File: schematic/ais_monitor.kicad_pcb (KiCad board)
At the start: 2 copper layers, 109.5 x 72.5 mm, 73 parts, among them J1 Power Input (12/24), J2 GPS, Q1 Q_NMOS_DGS, SW1 Mute, U1 TPS73701, U2 LM321, U3 ADP2302ARDZ, U4 Pico, U5 PAM8302AAD, U6 feather

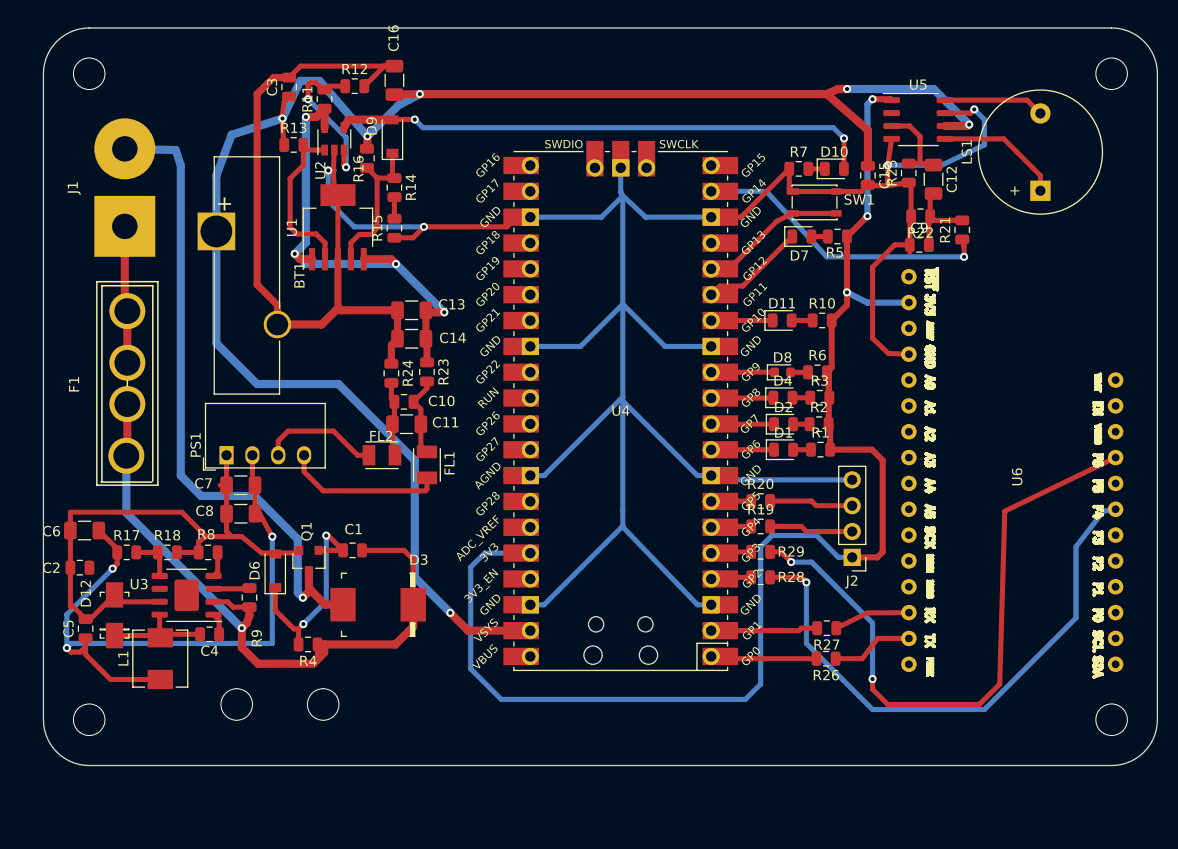
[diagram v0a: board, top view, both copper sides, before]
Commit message: more updates
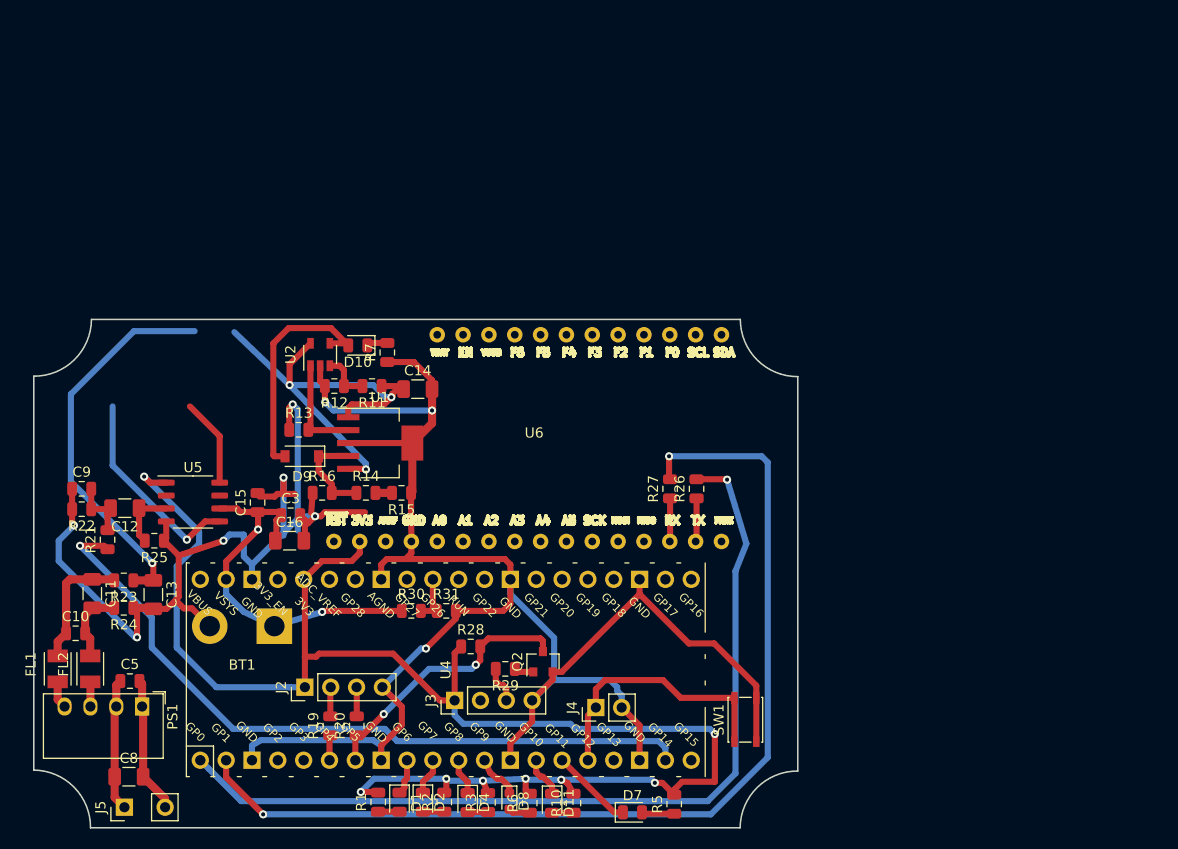
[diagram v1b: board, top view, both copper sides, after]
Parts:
- removed C1: 1u, Capacitor_SMD:C_0805_2012Metric
- removed C2: 22n, Capacitor_SMD:C_0805_2012Metric
- removed C4: 220n, Capacitor_SMD:C_0805_2012Metric
- removed C6, C7: 10u, Capacitor_SMD:C_1206_3216Metric
- removed D12: D, ais_monitor:DO-214AC
- removed D3: 40V, ais_monitor:DO-214AB
- removed D6: 5v6, Diode_SMD:D_SOD-123
- removed F1: Fuse, ais_monitor:BladeFuse-CarType
- removed J1: Power Input (12/24), Connector_Wire:SolderWirePad_1x02_P7.62mm_Drill2.5mm
- removed L1: 10u, Inductor_SMD:L_Sunlord_MWSA0518_5.4x5.2mm
- removed LS1: Speaker, Buzzer_Beeper:Buzzer_12x9.5RM7.6
- removed Q1: Q_NMOS_DGS, Package_TO_SOT_SMD:SOT-23
- removed R17: 56k, Resistor_SMD:R_0805_2012Metric
- removed R18, R4, R9: 10k, Resistor_SMD:R_0805_2012Metric
- removed R8: 47k, Resistor_SMD:R_0805_2012Metric
- removed U3: ADP2302ARDZ, pypilot_footprints:HSOP-8-1EP_3.9x4.9mm_P1.27mm_EP2.41x3.1mm
- added J3: GPS RS232, Connector_PinHeader_2.54mm:PinHeader_1x04_P2.54mm_Vertical, F.Cu at (132.4, 105.1)
- added J4: mute, Connector_PinHeader_2.54mm:PinHeader_1x02_P2.54mm_Vertical, F.Cu at (146.3, 105.8)
- added J5: IN5, Connector_PinHeader_2.54mm:PinHeader_1x02_P2.54mm_Vertical, F.Cu at (100.0, 115.6)
- added Q2: Q_NMOS_DGS, Package_TO_SOT_SMD:SOT-23, F.Cu at (141.1, 101.3)
- added R30: 100k, Resistor_SMD:R_0805_2012Metric, F.Cu at (128.2, 96.3)
- added R31: 100k, Resistor_SMD:R_0805_2012Metric, F.Cu at (131.6, 96.3)
- BT1: footprint Battery:Battery_Panasonic_CR2354-VCN_Vertical_CircularHoles -> Connector_Wire:SolderWirePad_1x02_P7.62mm_Drill2mm
- R28, R29: value 10k -> 2k4
- moved R21 89.4 mm to (98.3, 89.3)
- moved R22 87.3 mm to (95.8, 86.3)
- moved C12 85.8 mm to (100.0, 86.2), turned to 180 degrees
- moved C9 85.8 mm to (95.8, 84.3)
- moved R25 82.5 mm to (102.9, 89.4), turned to 180 degrees
- moved U5 80.6 mm to (106.7, 85.6)
- moved C15 68.1 mm to (113.0, 85.7), turned to 90 degrees
- moved D7 59.0 mm to (149.9, 116.1)
- moved R5 58.1 mm to (154.0, 115.3), turned to 90 degrees
- moved R1 55.6 mm to (124.9, 115.1), turned to 90 degrees
- moved J2 55.3 mm to (117.7, 103.8), turned to 90 degrees
- moved R10 53.4 mm to (144.1, 115.2), turned to 90 degrees
- moved D11 52.6 mm to (142.0, 115.2), turned to 270 degrees
- moved R2 52.3 mm to (131.4, 115.1), turned to 90 degrees
- moved R3 51.4 mm to (135.7, 115.1), turned to 90 degrees
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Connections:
- R28 pad 1: Net-(R28-Pad1) -> +3V3
- R28 pad 2: SLEEP -> RX1
- R29 pad 1: Net-(R29-Pad1) -> Net-(Q2-Pad1)
- R29 pad 2: LNA -> Net-(J3-Pad3)
- U4 pad 4: Net-(R28-Pad1) -> Net-(U4-Pad4)
- U4 pad 5: Net-(R29-Pad1) -> Net-(U4-Pad5)
- U6 pad 8: SLEEP -> Net-(U6-Pad8)
- U6 pad 9: LNA -> Net-(U6-Pad9)
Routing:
- net +BATT: track 171.3 -> 54.6 mm, vias 6 -> 3
- net RX0: track 10.5 -> 100.0 mm, vias 0 -> 2
- net TX0: track 11.7 -> 87.8 mm, vias 0 -> 1
- net Net-(C1-Pad1): track 69.9 -> 0.00 mm, vias 1 -> 0
- net Net-(D3-Pad2): track 64.0 -> 0.00 mm, vias 1 -> 0
- net LNA: track 62.5 -> 0.00 mm, vias 2 -> 0
- net GND: track 313.4 -> 257.3 mm, vias 4 -> 8
- net SLEEP: track 55.3 -> 0.00 mm, vias 1 -> 0
- net Net-(C5-Pad1): track 67.2 -> 13.0 mm, vias 3 -> 0
- net Net-(C2-Pad2): track 57.1 -> 13.4 mm
- net Net-(R21-Pad1): track 31.2 -> 71.5 mm
- net +5V: track 47.4 -> 84.4 mm
- net Net-(D10-Pad2): track 53.4 -> 22.8 mm, vias 2 -> 0
- net RX1: track 3.94 -> 26.7 mm, vias 0 -> 2
- net Net-(C1-Pad2): track 21.7 -> 0.00 mm, vias 2 -> 0
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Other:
- board size 109.5 x 72.5 mm -> 75.1 x 50 mm
